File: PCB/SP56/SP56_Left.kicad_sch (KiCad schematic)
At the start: 95 parts, among them J1 USB_C_Receptacle_USB2.0, J2 Conn_01x01_Male, J3 Conn_01x01_Male, J9 SM02B-SRSS-TB(LF)(SN), Q1 A03407, SW1 SW_PUSH, SW10 SW_PUSH, SW11 SW_PUSH, SW12 SW_PUSH, SW13 SW_PUSH, SW14 SW_PUSH, SW15 SW_PUSH, SW16 SW_PUSH, SW17 SW_PUSH, SW18 SW_PUSH, SW19 SW_PUSH, SW2 SW_PUSH, SW20 SW_PUSH, SW21 SW_PUSH, SW22 SW_PUSH, SW23 SW_PUSH, SW24 SW_PUSH, SW25 Rotary_Encoder_Switch, SW26 SW_PUSH, SW27 SW_PUSH, SW28 SW_PUSH, SW3 SW_PUSH, SW4 SW_PUSH, SW5 SW_PUSH, SW6 SW_PUSH, SW7 SW_PUSH, SW8 SW_PUSH, SW9 SW_PUSH, U1 LN2054Y42AMR, U2 E73-2G4M08S1C, U3 AP2112K-3.3, Y1 32.768kHz

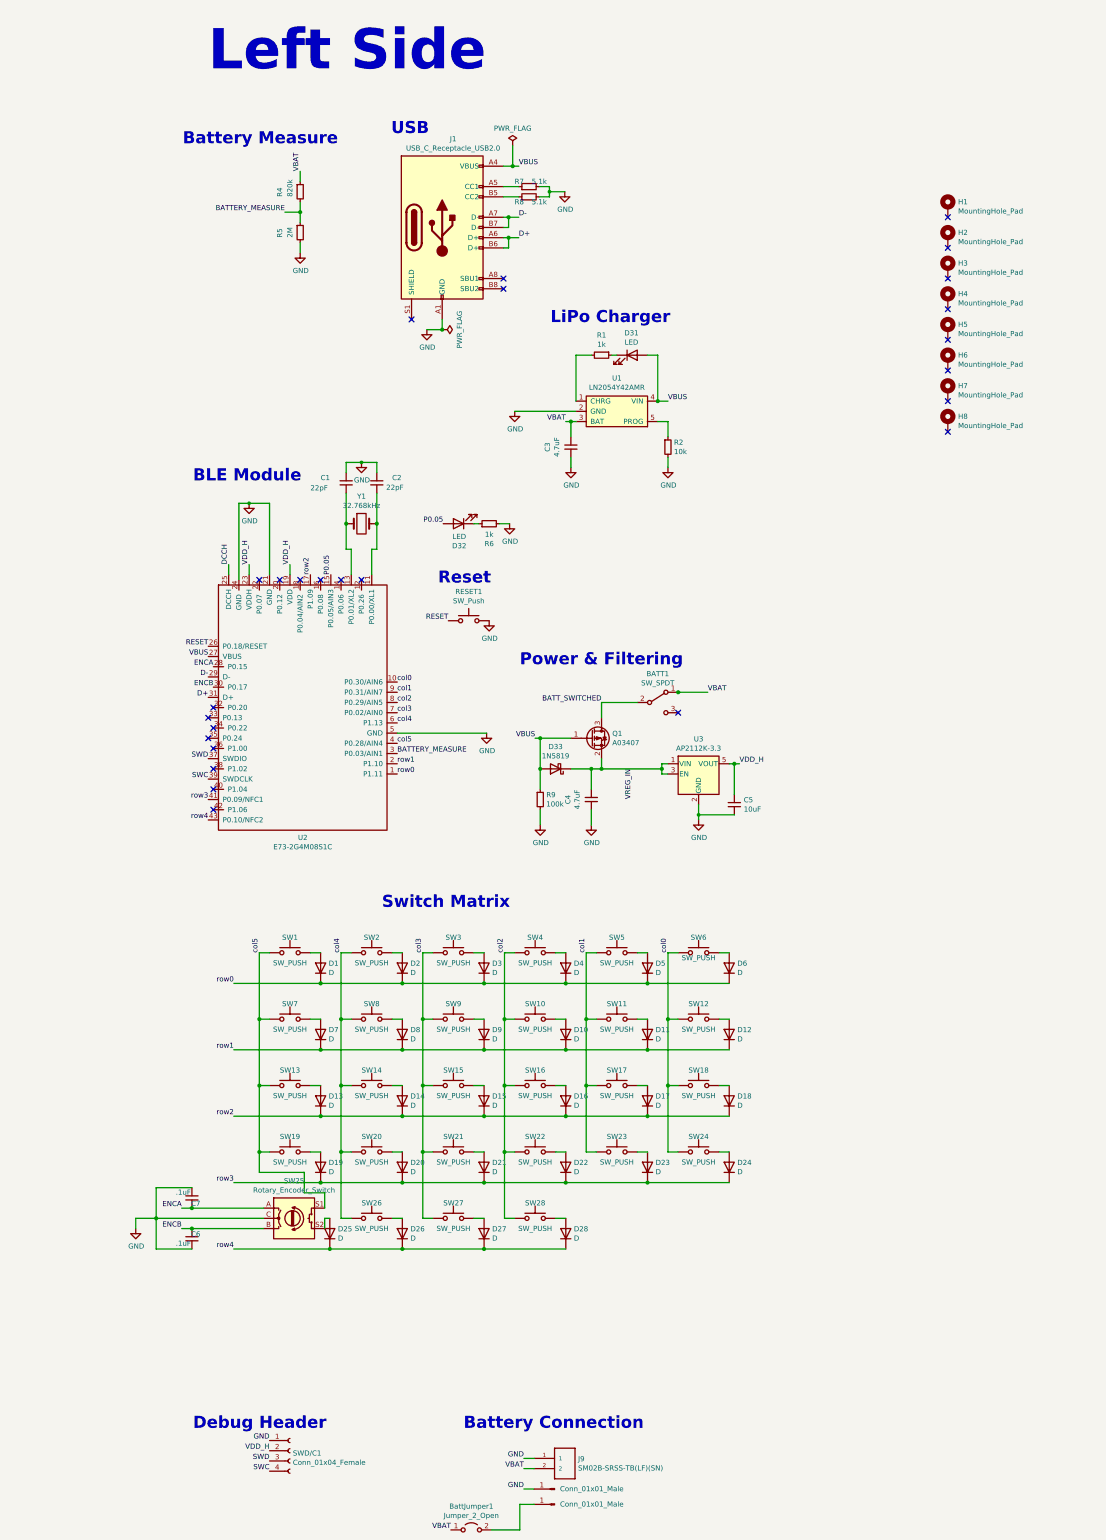
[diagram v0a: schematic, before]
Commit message: ready for jlc quote
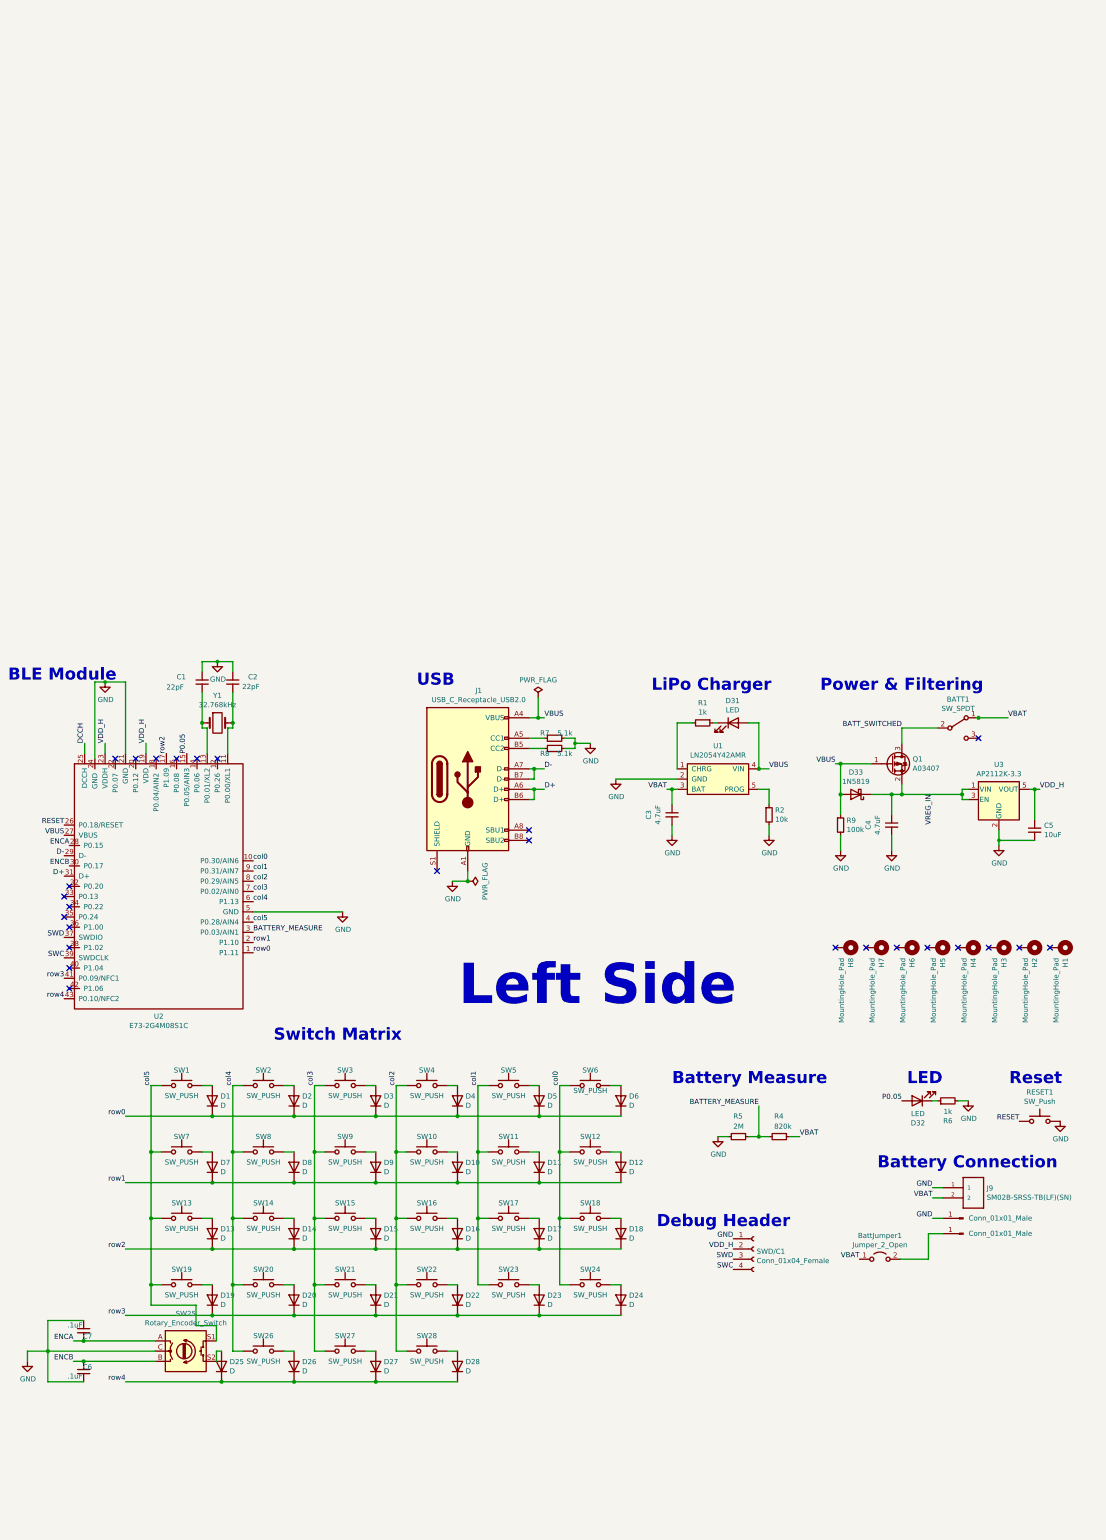
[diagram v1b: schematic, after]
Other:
- note added: "LED"
- company: (none) -> CO Boards
- title: (none) -> SP56
- moved on the sheet: BATT1, BattJumper1, C1, C2, C3, C4, C5, C6, C7, D1, D10, D11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
